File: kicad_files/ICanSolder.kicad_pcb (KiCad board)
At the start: 2 copper layers, 40 x 48.2 mm, 6 parts

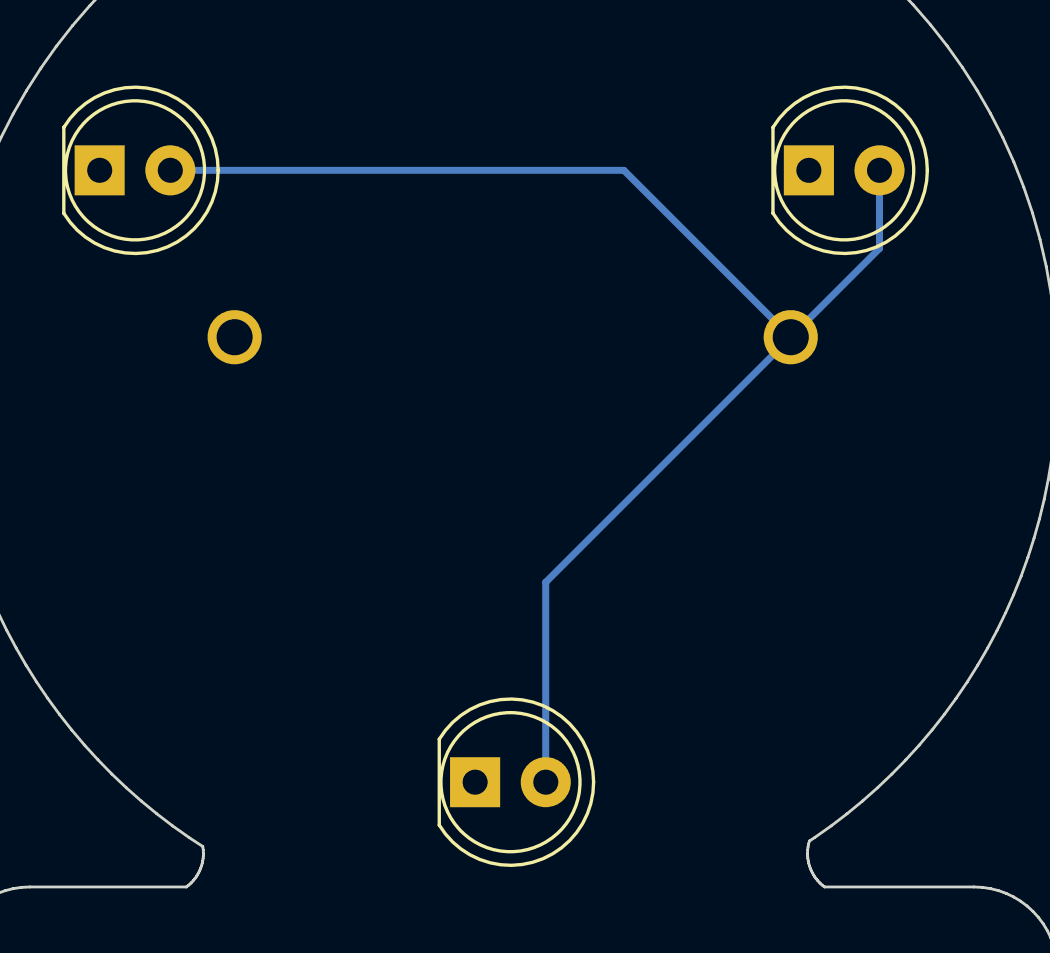
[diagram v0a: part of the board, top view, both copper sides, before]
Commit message: fixed minor errors
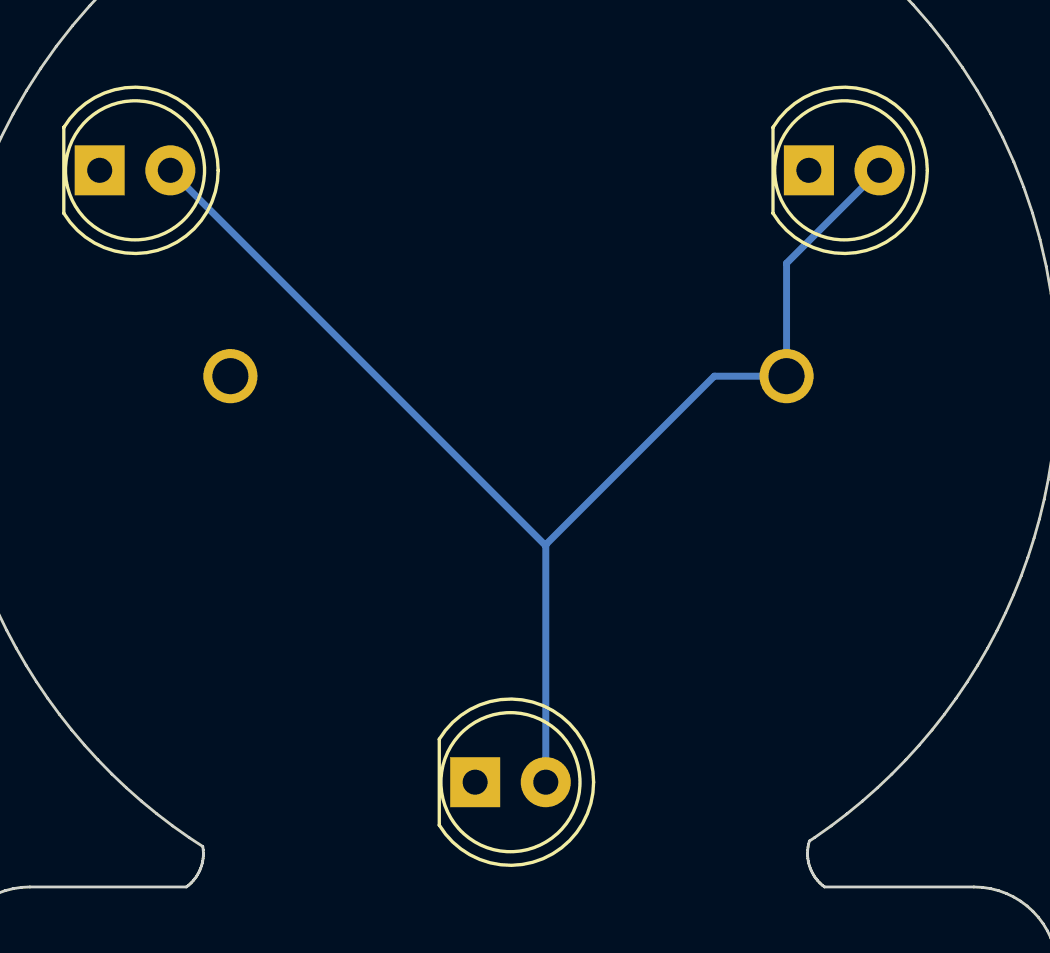
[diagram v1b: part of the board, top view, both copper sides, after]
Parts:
- moved BT1 1.41 mm to (179.3, 115.4)
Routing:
- net VCC: track 51.8 -> 47.6 mm
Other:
- board text added: "V2.1"
- board text removed: "V2.0"
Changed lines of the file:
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@@
-(kicad_pcb (version 20171130) (host pcbnew 5.1.6)
+(kicad_pcb (version 20171130) (host pcbnew 5.1.9)
   (general
     (thickness 1.6)
     (drawings 8)
-    (tracks 6)
+    (tracks 7)
     (zones 0)
     (modules 6)
@@
   )
   (module Batteries:BATTCOM_20MM_PTH (layer B.Cu)
-    (at 179.5 114)
+    (at 179.34832 115.4)
     (descr "20MM (CR2032) COIN CELL BATTERY HOLDER - PTH")
     (tags "20MM (CR2032) COIN CELL BATTERY HOLDER - PTH")
@@
   )
   (gr_text + (at 194.5 109.35) (layer B.SilkS)
-    (effects (font (size 0.5 0.5) (thickness 0.125)) (justify mirror))
+    (effects (font (size 1 1) (thickness 0.125)) (justify mirror))
   )
   (gr_text + (at 169 109.35) (layer B.SilkS)
-    (effects (font (size 0.5 0.5) (thickness 0.125)) (justify mirror))
+    (effects (font (size 1 1) (thickness 0.125)) (justify mirror))
   )
   (gr_text + (at 182.5 131.35) (layer B.SilkS)
-    (effects (font (size 0.5 0.5) (thickness 0.125)) (justify mirror))
-  )
-  (gr_text "CC-BY-SA 4.0" (at 189.4 129.5) (layer B.SilkS)
+    (effects (font (size 1 1) (thickness 0.125)) (justify mirror))
+  )
+  (gr_text "CC-BY-SA 4.0" (at 172.8 129.5) (layer B.SilkS)
     (effects (font (size 0.8 0.8) (thickness 0.11)) (justify mirror))
   )
-  (gr_text "Binary Kitchen" (at 189.5 127.85) (layer B.SilkS)
+  (gr_text "Binary Kitchen" (at 172.9 127.85) (layer B.SilkS)
     (effects (font (size 0.8 0.8) (thickness 0.11)) (justify mirror))
   )
-  (gr_text V2.0 (at 185.5 126.25) (layer B.SilkS)
-    (effects (font (size 0.5 0.5) (thickness 0.11)) (justify mirror))
-  )
-  (gr_text "I can solder" (at 189.2 125.15) (layer B.SilkS)
+  (gr_text V2.1 (at 186.6 128.7) (layer B.SilkS)
+    (effects (font (size 0.55 0.55) (thickness 0.11)) (justify mirror))
+  )
+  (gr_text "I can solder" (at 190.3 127.55) (layer B.SilkS)
     (effects (font (size 1 1) (thickness 0.25)) (justify mirror))
   )
-  (segment (start 182.54 122.8091) (end 191.3491 114) (width 0.25) (layer B.Cu) (net 2))
-  (segment (start 182.54 130) (end 182.54 122.8091) (width 0.25) (layer B.Cu) (net 2))
-  (segment (start 194.54 110.8091) (end 191.3491 114) (width 0.25) (layer B.Cu) (net 2))
-  (segment (start 194.54 108) (end 194.54 110.8091) (width 0.25) (layer B.Cu) (net 2))
-  (segment (start 185.3491 108) (end 191.3491 114) (width 0.25) (layer B.Cu) (net 2))
-  (segment (start 169.04 108) (end 185.3491 108) (width 0.25) (layer B.Cu) (net 2))
+  (segment (start 182.54 121.5) (end 169.04 108) (width 0.25) (layer B.Cu) (net 2))
+  (segment (start 182.54 130) (end 182.54 121.5) (width 0.25) (layer B.Cu) (net 2))
+  (segment (start 182.54 121.5) (end 182.54 121.46) (width 0.25) (layer B.Cu) (net 2))
+  (segment (start 188.6 115.4) (end 191.19742 115.4) (width 0.25) (layer B.Cu) (net 2))
+  (segment (start 182.54 121.46) (end 188.6 115.4) (width 0.25) (layer B.Cu) (net 2))
+  (segment (start 191.19742 111.34258) (end 194.54 108) (width 0.25) (layer B.Cu) (net 2))
+  (segment (start 191.19742 115.4) (end 191.19742 111.34258) (width 0.25) (layer B.Cu) (net 2))
   (zone (net 1) (net_name GND) (layer F.Cu) (hatch edge 0.508)
     (connect_pads (clearance 0.508))
